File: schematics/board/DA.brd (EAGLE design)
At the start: 82 x 82 mm, 48 parts, among them Q24 Q24

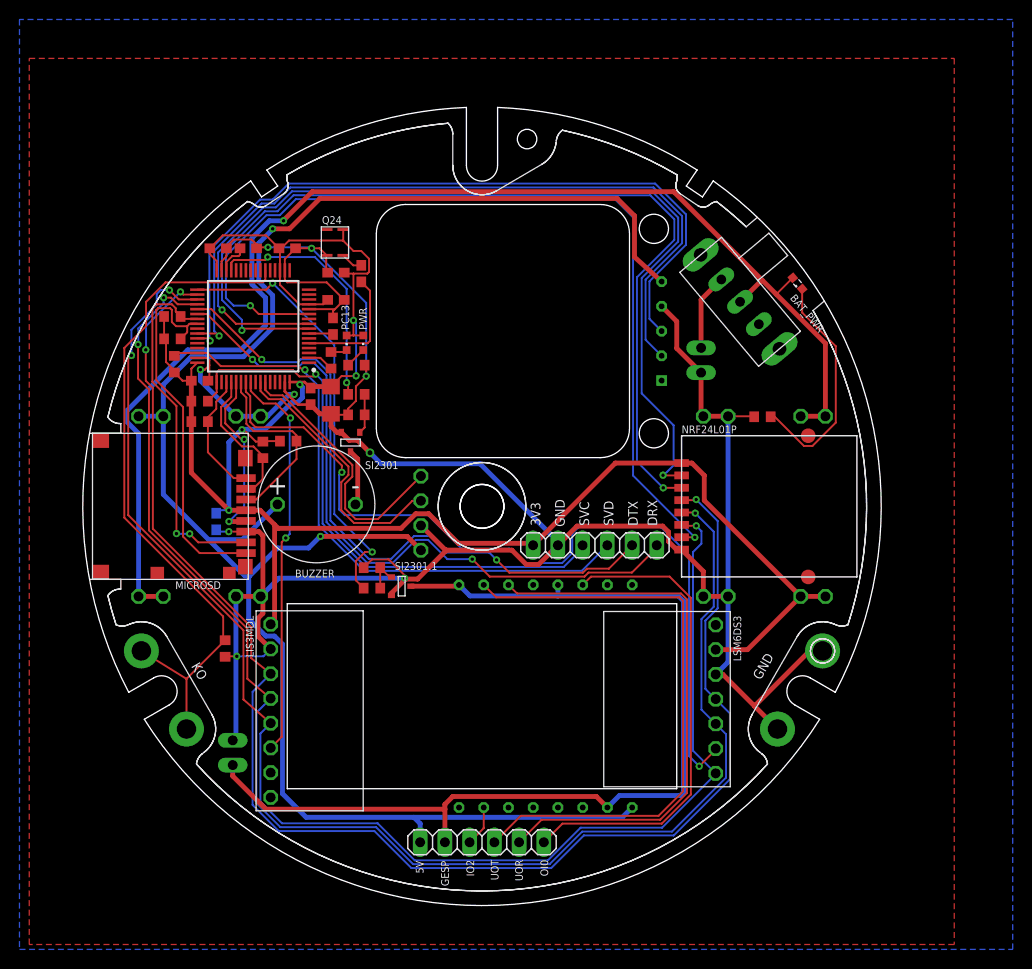
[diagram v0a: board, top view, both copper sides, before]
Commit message: Еще раз проверил все платы и подготовил для производства в Резоните
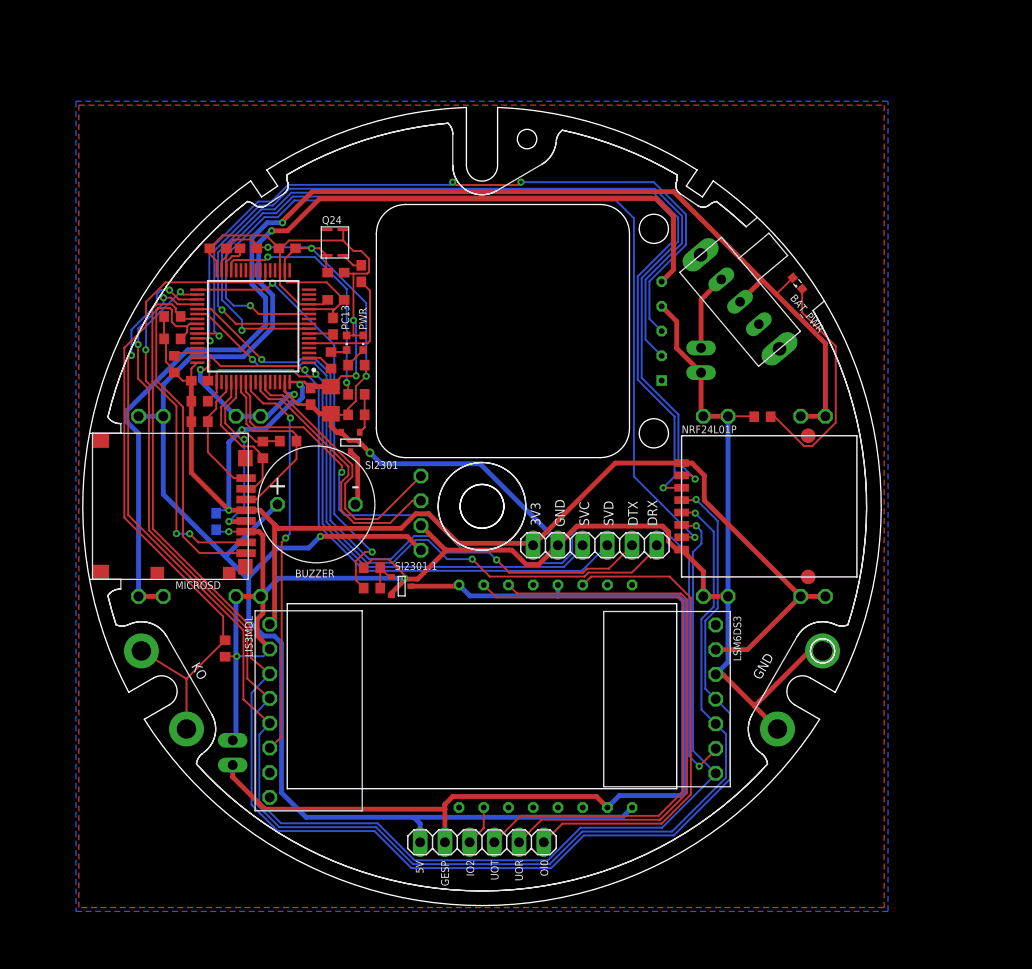
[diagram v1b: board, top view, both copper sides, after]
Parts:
- moved LIS3MDL 0.10 mm to (23.2, 20.0)
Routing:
- net 5V: track 191.3 -> 193.6 mm
- net CS_NRF: track 97.8 -> 98.6 mm
- net GPS_RX: track 77.9 -> 78.3 mm, vias 1 -> 3
